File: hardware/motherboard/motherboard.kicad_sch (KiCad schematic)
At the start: 80 parts, among them J1 JST-VH, J2 USB C 2.0, J3 JST-VH, J4 JST-PH, J5 IMU Connector, Q1 TSM7P06CP_ROG, Q2 TSM7P06CP_ROG, SW10 B, SW11 X, SW12 Y, SW13 Start, SW14 Select, SW2 Reset, SW3 A, SW4 B, SW5 LB, SW6 RB, SW7 X, SW8 Y, SW9 A, U1 ESP32-S3-WROOM-1, U2 TPS75533KTTRG3, U3 TLV75709PDBV, U4 MCP73831-2-OT

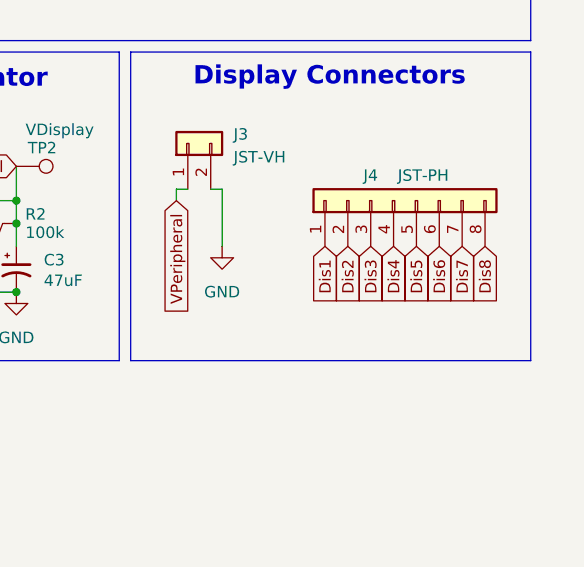
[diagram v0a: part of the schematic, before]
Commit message: Started Motherboard PCB Layout
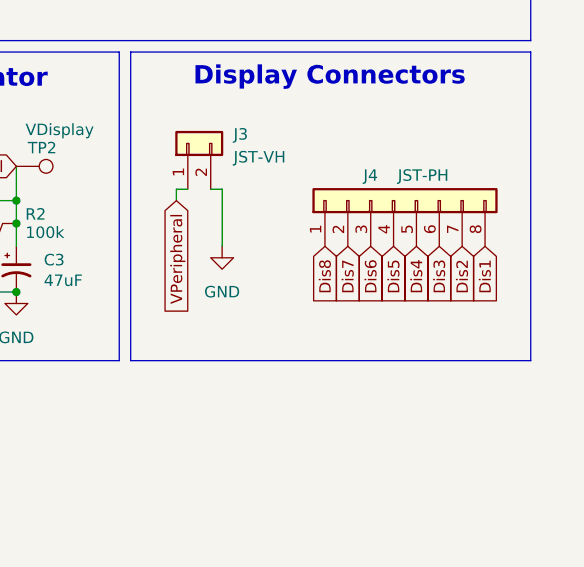
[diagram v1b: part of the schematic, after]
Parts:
- J1: footprint Connector_JST:JST_VH_B2P-VH-FB-B_1x02_P3.96mm_Vertical -> Connector_JST:JST_VH_B2PS-VH_1x02_P3.96mm_Horizontal
- J4: footprint Connector_JST:JST_PH_B8B-PH-SM4-TB_1x08-1MP_P2.00mm_Vertical -> Connector_JST:JST_PH_S8B-PH-K_1x08_P2.00mm_Horizontal
- J5: footprint (none) -> Connector_PinHeader_2.54mm:PinHeader_1x08_P2.54mm_Vertical
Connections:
- net Dis1: now also J4.8 (Pin_8); no longer J4.1 (Pin_1)
- net Dis2: now also J4.7 (Pin_7); no longer J4.2 (Pin_2)
- net Dis3: now also J4.6 (Pin_6); no longer J4.3 (Pin_3)
- net Dis4: now also J4.5 (Pin_5); no longer J4.4 (Pin_4)
- net Dis5: now also J4.4 (Pin_4); no longer J4.5 (Pin_5)
- net Dis6: now also J4.3 (Pin_3); no longer J4.6 (Pin_6)
- net Dis7: now also J4.2 (Pin_2); no longer J4.7 (Pin_7)
- net Dis8: now also J4.1 (Pin_1); no longer J4.8 (Pin_8)
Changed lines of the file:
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@@
 	(wire
 		(pts
+			(xy 118.11 180.34) (xy 119.38 180.34)
+		)
+		(stroke
+			(width 0)
+			(type default)
+		)
+	)
+	(wire
+		(pts
 			(xy 72.39 69.85) (xy 73.66 69.85)
 		)
@@
 	(wire
 		(pts
-			(xy 118.11 180.34) (xy 119.38 180.34)
-		)
-		(stroke
-			(width 0)
-			(type default)
-		)
-	)
-	(wire
-		(pts
 			(xy 91.44 31.75) (xy 91.44 33.02)
 		)
@@
 	(global_label "Dis7"
 		(shape input)
-		(at 275.59 152.4 270)
+		(at 262.89 152.4 270)
 		(fields_autoplaced yes)
 		(effects
@@
 		)
 		(property "Intersheetrefs" "${INTERSHEET_REFS}"
-			(at 275.59 159.4976 90)
+			(at 262.89 159.4976 90)
 			(effects
 				(font
@@
 	(global_label "Dis3"
 		(shape input)
-		(at 265.43 152.4 270)
+		(at 273.05 152.4 270)
 		(fields_autoplaced yes)
 		(effects
@@
 		)
 		(property "Intersheetrefs" "${INTERSHEET_REFS}"
-			(at 265.43 159.4976 90)
+			(at 273.05 159.4976 90)
 			(effects
 				(font
@@
 	(global_label "Dis2"
 		(shape input)
-		(at 262.89 152.4 270)
+		(at 275.59 152.4 270)
 		(fields_autoplaced yes)
 		(effects
@@
 		)
 		(property "Intersheetrefs" "${INTERSHEET_REFS}"
-			(at 262.89 159.4976 90)
+			(at 275.59 159.4976 90)
 			(effects
 				(font
@@
 	(global_label "Dis6"
 		(shape input)
-		(at 273.05 152.4 270)
+		(at 265.43 152.4 270)
 		(fields_autoplaced yes)
 		(effects
@@
 		)
 		(property "Intersheetrefs" "${INTERSHEET_REFS}"
-			(at 273.05 159.4976 90)
+			(at 265.43 159.4976 90)
 			(effects
 				(font
@@
 	(global_label "Dis4"
 		(shape input)
-		(at 267.97 152.4 270)
+		(at 270.51 152.4 270)
 		(fields_autoplaced yes)
 		(effects
@@
 		)
 		(property "Intersheetrefs" "${INTERSHEET_REFS}"
-			(at 267.97 159.4976 90)
+			(at 270.51 159.4976 90)
 			(effects
 				(font
@@
 	(global_label "Dis5"
 		(shape input)
-		(at 270.51 152.4 270)
+		(at 267.97 152.4 270)
 		(fields_autoplaced yes)
 		(effects
@@
 		)
 		(property "Intersheetrefs" "${INTERSHEET_REFS}"
-			(at 270.51 159.4976 90)
+			(at 267.97 159.4976 90)
 			(effects
 				(font
@@
 	(global_label "Dis1"
 		(shape input)
-		(at 260.35 152.4 270)
+		(at 278.13 152.4 270)
 		(fields_autoplaced yes)
 		(effects
@@
 		)
 		(property "Intersheetrefs" "${INTERSHEET_REFS}"
-			(at 260.35 159.4976 90)
+			(at 278.13 159.4976 90)
 			(effects
 				(font
@@
 	(global_label "Dis8"
 		(shape input)
-		(at 278.13 152.4 270)
+		(at 260.35 152.4 270)
 		(fields_autoplaced yes)
 		(effects
@@
 		)
 		(property "Intersheetrefs" "${INTERSHEET_REFS}"
-			(at 278.13 159.4976 90)
+			(at 260.35 159.4976 90)
 			(effects
 				(font
@@
 			)
 		)
-		(property "Footprint" ""
+		(property "Footprint" "Connector_PinHeader_2.54mm:PinHeader_1x08_P2.54mm_Vertical"
 			(at 30.48 107.95 0)
 			(effects
@@
 			)
 		)
-		(property "Footprint" "Connector_JST:JST_VH_B2P-VH-FB-B_1x02_P3.96mm_Vertical"
+		(property "Footprint" "Connector_JST:JST_VH_B2PS-VH_1x02_P3.96mm_Horizontal"
 			(at 17.78 121.92 0)
 			(effects
@@
 			)
 		)
-		(property "Footprint" "Connector_JST:JST_PH_B8B-PH-SM4-TB_1x08-1MP_P2.00mm_Vertical"
+		(property "Footprint" "Connector_JST:JST_PH_S8B-PH-K_1x08_P2.00mm_Horizontal"
 			(at 267.97 147.32 0)
 			(effects
